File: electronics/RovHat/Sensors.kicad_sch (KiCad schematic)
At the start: 14 parts, among them J201 ADS1115, J202 ANALOG INPUT, J203 GYRO

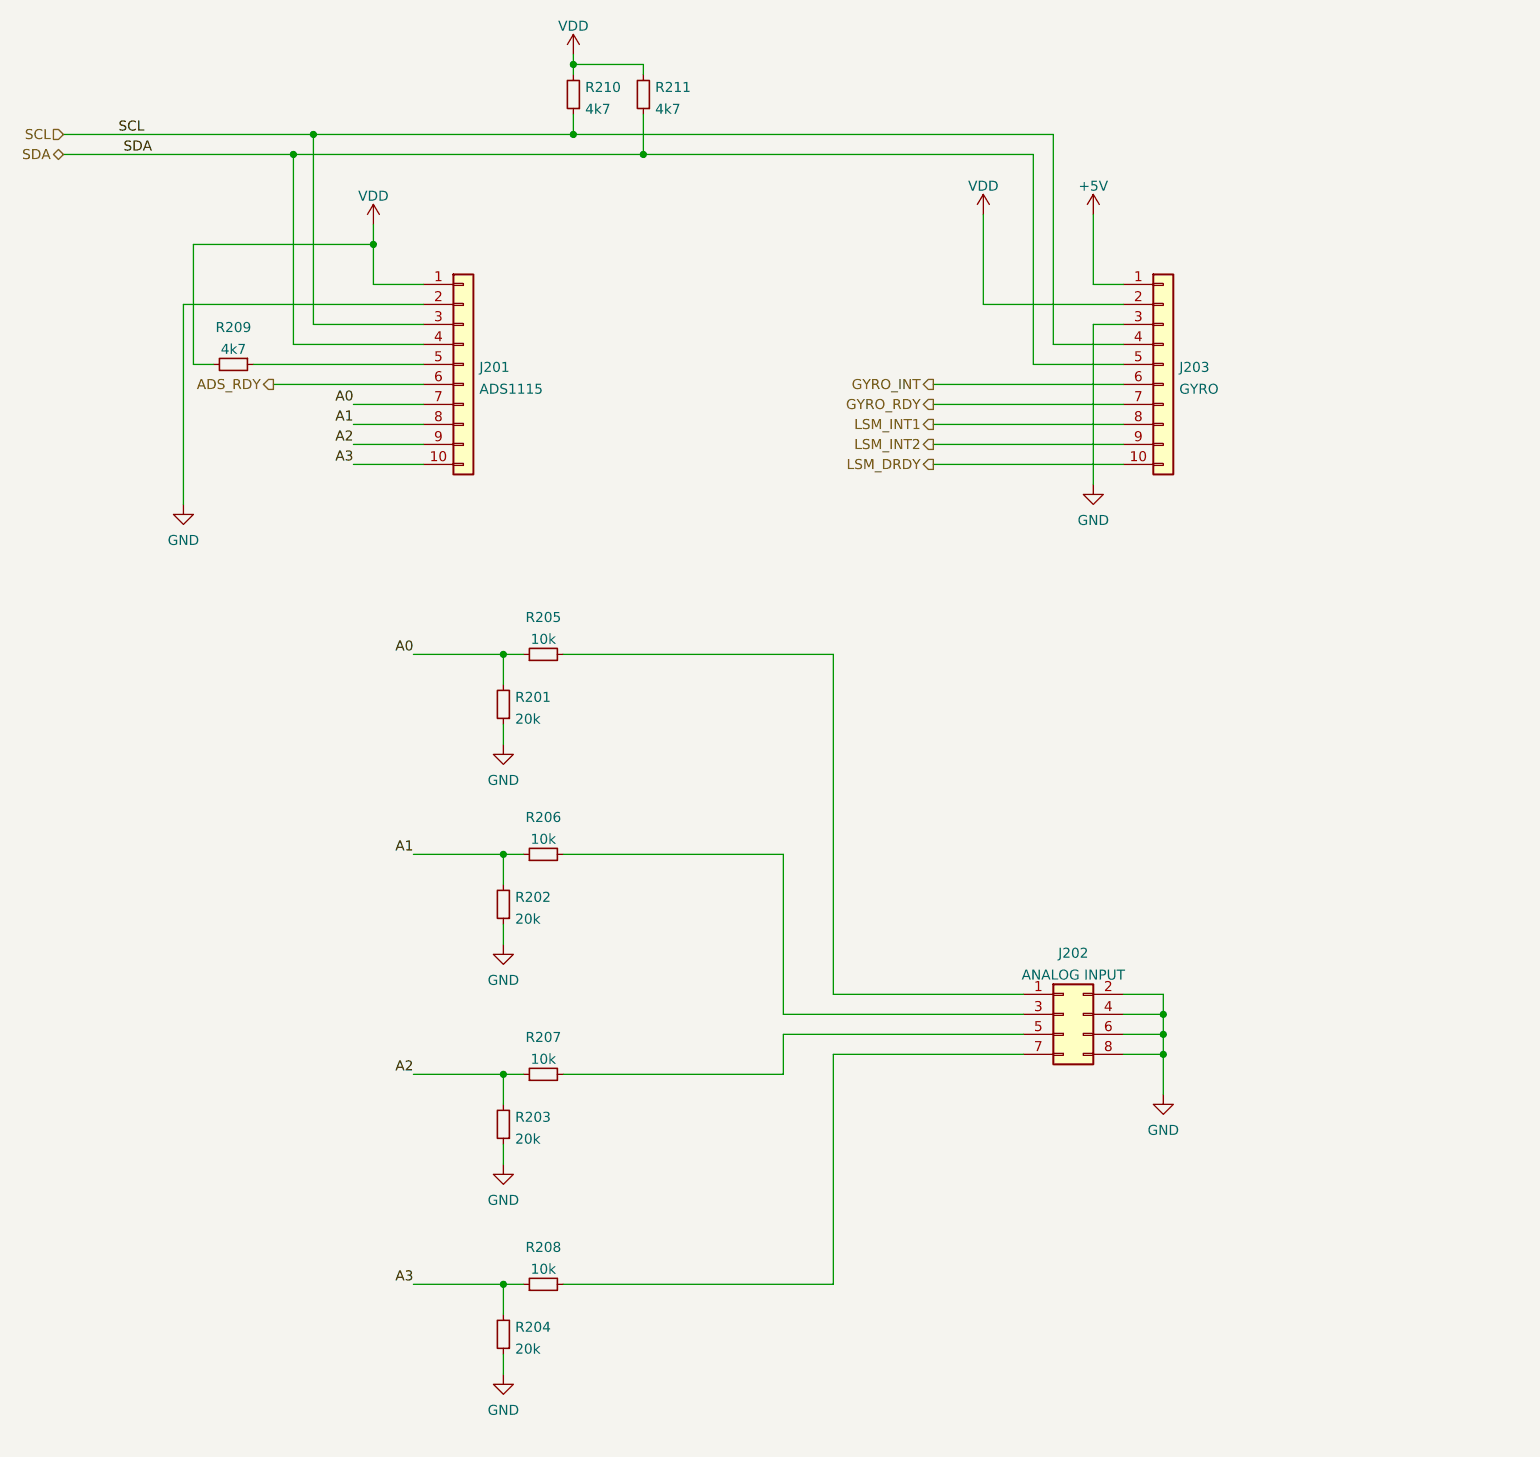
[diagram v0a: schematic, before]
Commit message: Fabrication commit 2
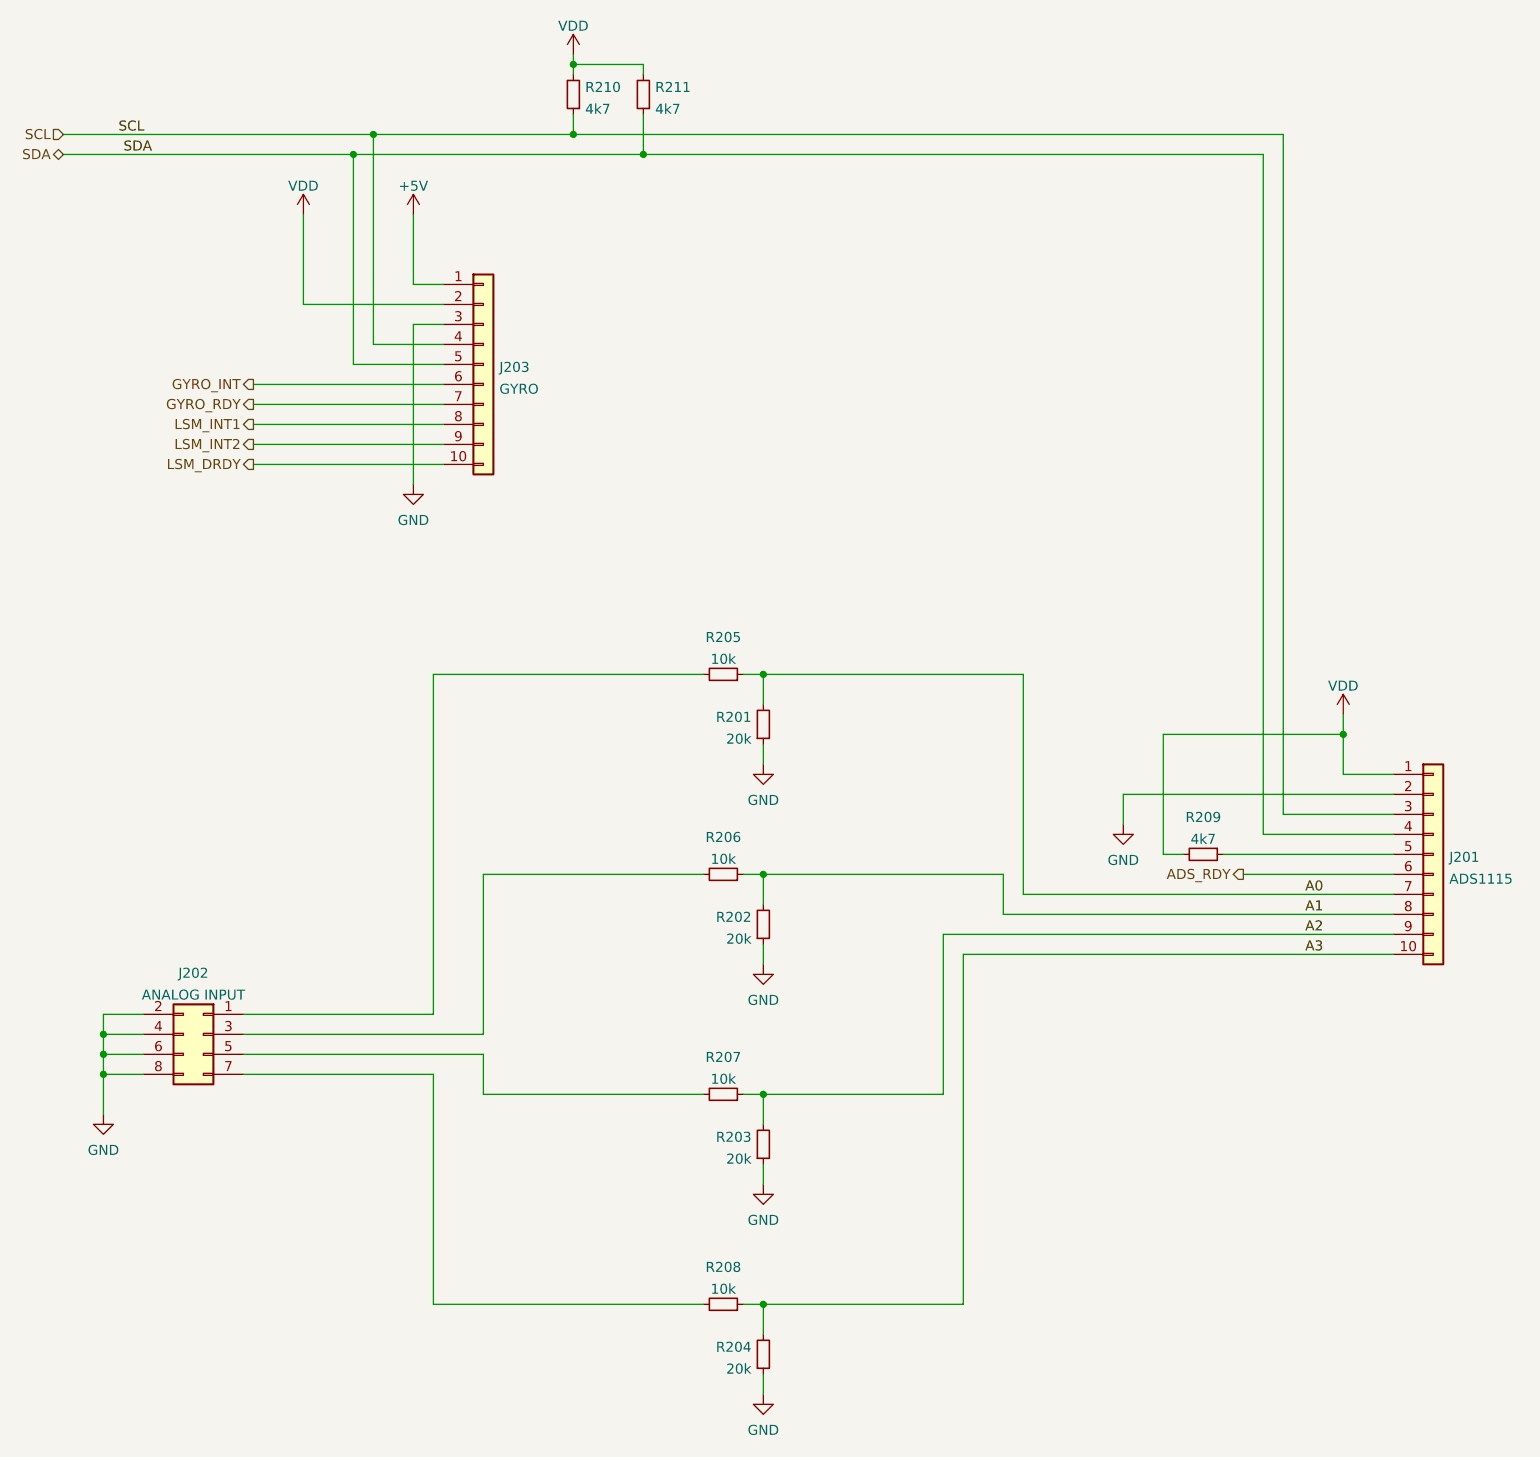
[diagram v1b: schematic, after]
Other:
- company: (none) -> Findersee
- title: (none) -> ROV RPI PICO HAT
- moved on the sheet: J201, J202, J203, R201, R202, R203, R204, R205, R206, R207, R208, R209
